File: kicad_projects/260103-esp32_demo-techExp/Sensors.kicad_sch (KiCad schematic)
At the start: 0 parts

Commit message: regular
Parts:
- added C15, C16, C18, C20: 100n, Capacitor_SMD:C_0805_2012Metric, symbol Device:C
- added MK1: CMC-5042PF-AC, esp32_demo_footprints:CUI_CMC-5042PF-AC, symbol CMC-5042PF-AC:CMC-5042PF-AC
- added Q1: TEMT6000X01, esp32_demo_footprints:TRANS_TEMT6000X01, symbol TEMT6000X01:TEMT6000X01
- added R23, R30: 10k, Resistor_SMD:R_0805_2012Metric, symbol Device:R
- added R24, R25: 4k7, Resistor_SMD:R_0805_2012Metric, symbol Device:R
- added R26, R28: 2k, Resistor_SMD:R_0805_2012Metric, symbol Device:R
- added R27, R29: 1M, Resistor_SMD:R_0805_2012Metric, symbol Device:R
- added R31: 100k, Resistor_SMD:R_0805_2012Metric, symbol Device:R
- added U7: BME280, esp32_demo_footprints:PSON65P250X250X100-8N, symbol BME280:BME280
- added U8: MAX4466EXK, esp32_demo_footprints:SOT65P210X110-5N, symbol MAX4466EXK:MAX4466EXK
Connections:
- new net: C16.2, R26.1, R28.2
- new net: MK1.OUT, R27.1, R28.1, R29.2, U8.1 (IN+)
- new net: C20.1, R30.2, R31.1, U8.3 (IN-)
- new net +3.3V: C15.1, C18.1, R23.1, R24.1, R25.1, R26.2, R27.2, U7.2 (CSB), U7.6 (VDDIO), U7.8 (VDD), U8.5 (VCC)
- new net GND: C15.2, C16.1, C18.2, MK1.GND, Q1.1, R29.1, R30.1, U7.1 (GND), U7.5 (SDO), U7.7 (GND), U8.2 (GND)
- new net MIC_OUT: C20.2, R31.2, U8.4 (OUT)
- new net PHOTO_C: Q1.3, R23.2
- new net SCL: R24.2, U7.4 (SCK)
- new net SDA: R25.2, U7.3 (SDI)
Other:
- note added: "BME280"
- note added: "Micophone and amplifier"
- note added: "Photo sensor"
- note added: "for SDO is grounded, the address is 0x76"

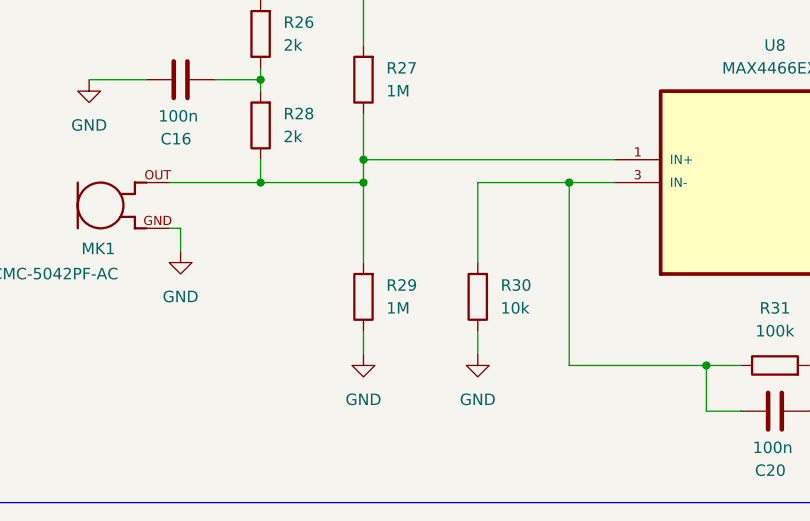
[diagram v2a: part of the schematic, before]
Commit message: regular
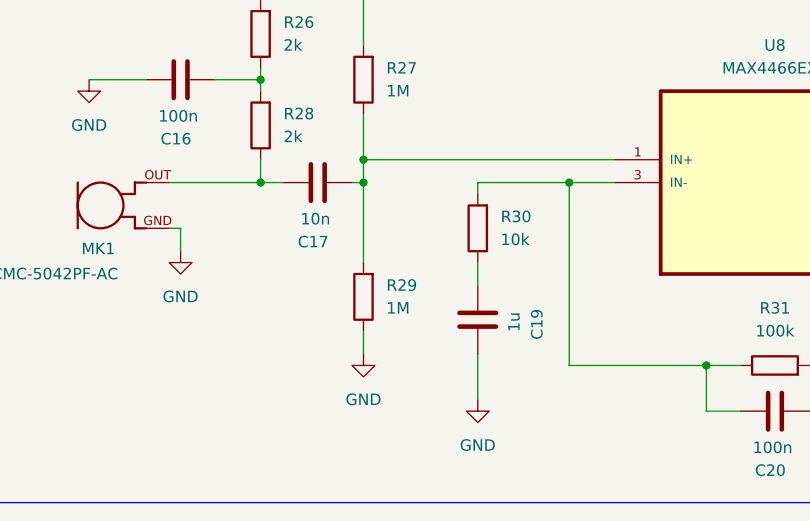
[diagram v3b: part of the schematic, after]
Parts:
- added C17: 10n, Capacitor_SMD:C_0805_2012Metric, symbol Device:C
- added C19: 1u, Capacitor_SMD:C_0805_2012Metric, symbol Device:C
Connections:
- net GND: now also C19.1; no longer R30.1
- net at R27.1, R29.2, U8.1 (IN+): now also C17.2; no longer MK1.OUT, R28.1
- new net: C17.1, MK1.OUT, R28.1
- new net: C19.2, R30.1
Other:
- moved on the sheet: R30
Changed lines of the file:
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@@
+	)
+	(junction
+		(at 176.53 127)
+		(diameter 0)
+		(color 0 0 0 0)
 	)
 	(junction
@@
 	)
 	(junction
-		(at 165.1 127)
-		(diameter 0)
-		(color 0 0 0 0)
-	)
-	(junction
 		(at 250.19 119.38)
 		(diameter 0)
@@
 	)
 	(junction
-		(at 176.53 127)
+		(at 165.1 127)
 		(diameter 0)
 		(color 0 0 0 0)
@@
 	(wire
 		(pts
+			(xy 176.53 127) (xy 176.53 135.89)
+		)
+		(stroke
+			(width 0)
+			(type default)
+		)
+	)
+	(wire
+		(pts
 			(xy 156.21 132.08) (xy 156.21 134.62)
 		)
@@
 	(wire
 		(pts
-			(xy 165.1 127) (xy 176.53 127)
-		)
-		(stroke
-			(width 0)
-			(type default)
-		)
-	)
-	(wire
-		(pts
 			(xy 97.79 54.61) (xy 97.79 52.07)
 		)
@@
 	(wire
 		(pts
-			(xy 189.23 135.89) (xy 189.23 127)
+			(xy 189.23 128.27) (xy 189.23 127)
 		)
 		(stroke
@@
 	(wire
 		(pts
+			(xy 165.1 127) (xy 167.64 127)
+		)
+		(stroke
+			(width 0)
+			(type default)
+		)
+	)
+	(wire
+		(pts
 			(xy 97.79 72.39) (xy 97.79 74.93)
 		)
@@
 	(wire
 		(pts
-			(xy 176.53 127) (xy 176.53 135.89)
-		)
-		(stroke
-			(width 0)
-			(type default)
-		)
-	)
-	(wire
-		(pts
 			(xy 154.94 127) (xy 165.1 127)
 		)
@@
 	(wire
 		(pts
-			(xy 189.23 143.51) (xy 189.23 146.05)
+			(xy 189.23 135.89) (xy 189.23 138.43)
 		)
 		(stroke
@@
 	(wire
 		(pts
+			(xy 189.23 151.13) (xy 189.23 146.05)
+		)
+		(stroke
+			(width 0)
+			(type default)
+		)
+	)
+	(wire
+		(pts
 			(xy 176.53 143.51) (xy 176.53 146.05)
 		)
@@
 		(pts
 			(xy 214.63 152.4) (xy 214.63 147.32)
+		)
+		(stroke
+			(width 0)
+			(type default)
+		)
+	)
+	(wire
+		(pts
+			(xy 175.26 127) (xy 176.53 127)
 		)
 		(stroke
@@
 	(symbol
 		(lib_id "power:GND")
-		(at 189.23 146.05 0)
+		(at 189.23 151.13 0)
 		(unit 1)
 		(exclude_from_sim no)
@@
 		(fields_autoplaced yes)
 		(property "Reference" "#PWR049"
-			(at 189.23 152.4 0)
+			(at 189.23 157.48 0)
 			(effects
 				(font
@@
 		)
 		(property "Value" "GND"
+			(at 189.23 156.21 0)
+			(effects
+				(font
+					(size 1.27 1.27)
+				)
+			)
+		)
+		(property "Footprint" ""
 			(at 189.23 151.13 0)
 			(effects
@@
 					(size 1.27 1.27)
 				)
-			)
-		)
-		(property "Footprint" ""
-			(at 189.23 146.05 0)
-			(effects
-				(font
-					(size 1.27 1.27)
-				)
 				(hide yes)
 			)
 		)
 		(property "Datasheet" ""
-			(at 189.23 146.05 0)
+			(at 189.23 151.13 0)
 			(effects
 				(font
@@
 		)
 		(property "Description" "Power symbol creates a global label with name \"GND\" , ground"
-			(at 189.23 146.05 0)
+			(at 189.23 151.13 0)
 			(effects
 				(font
@@
 	)
 	(symbol
+		(lib_id "Device:C")
+		(at 171.45 127 90)
+		(unit 1)
+		(exclude_from_sim no)
+		(in_bom yes)
+		(on_board yes)
+		(dnp no)
+		(property "Reference" "C17"
+			(at 170.942 133.604 90)
+			(effects
+				(font
+					(size 1.27 1.27)
+				)
+			)
+		)
+		(property "Value" "10n"
+			(at 171.196 131.064 90)
+			(effects
+				(font
+					(size 1.27 1.27)
+				)
+			)
+		)
+		(property "Footprint" "Capacitor_SMD:C_0805_2012Metric"
+			(at 175.26 126.0348 0)
+			(effects
+				(font
+					(size 1.27 1.27)
+				)
+				(hide yes)
+			)
+		)
+		(property "Datasheet" "~"
+			(at 171.45 127 0)
+			(effects
+				(font
+					(size 1.27 1.27)
+				)
+				(hide yes)
+			)
+		)
+		(property "Description" "Unpolarized capacitor"
+			(at 171.45 127 0)
+			(effects
+				(font
+					(size 1.27 1.27)
+				)
+				(hide yes)
+			)
+		)
+		(pin "1"
+		)
+		(pin "2"
+		)
+		(instances
+			(project "260103-esp32_demo-techExp"
+				(path "/2d426d0b-8cb5-4c97-a124-03a3dc3f5ac0/c970ae5e-5c0d-4bfd-b9e3-3da90c7c28e6/aa4b4bc5-e6e9-40a7-8829-625116ed9b5f"
+					(reference "C17")
+					(unit 1)
+				)
+			)
+		)
+	)
+	(symbol
+		(lib_id "Device:C")
+		(at 189.23 142.24 180)
+		(unit 1)
+		(exclude_from_sim no)
+		(in_bom yes)
+		(on_board yes)
+		(dnp no)
+		(property "Reference" "C19"
+			(at 195.834 142.748 90)
+			(effects
+				(font
+					(size 1.27 1.27)
+				)
+			)
+		)
+		(property "Value" "1u"
+			(at 193.294 142.494 90)
+			(effects
+				(font
+					(size 1.27 1.27)
+				)
+			)
+		)
+		(property "Footprint" "Capacitor_SMD:C_0805_2012Metric"
+			(at 188.2648 138.43 0)
+			(effects
+				(font
+					(size 1.27 1.27)
+				)
+				(hide yes)
+			)
+		)
+		(property "Datasheet" "~"
+			(at 189.23 142.24 0)
+			(effects
+				(font
+					(size 1.27 1.27)
+				)
+				(hide yes)
+			)
+		)
+		(property "Description" "Unpolarized capacitor"
+			(at 189.23 142.24 0)
+			(effects
+				(font
+					(size 1.27 1.27)
+				)
+				(hide yes)
+			)
+		)
+		(pin "1"
+		)
+		(pin "2"
+		)
+		(instances
+			(project "260103-esp32_demo-techExp"
+				(path "/2d426d0b-8cb5-4c97-a124-03a3dc3f5ac0/c970ae5e-5c0d-4bfd-b9e3-3da90c7c28e6/aa4b4bc5-e6e9-40a7-8829-625116ed9b5f"
+					(reference "C19")
+					(unit 1)
+				)
+			)
+		)
+	)
+	(symbol
 		(lib_id "Device:R")
 		(at 165.1 120.65 180)
@@
 	(symbol
 		(lib_id "Device:R")
-		(at 189.23 139.7 180)
+		(at 189.23 132.08 180)
 		(unit 1)
 		(exclude_from_sim no)
@@
 		(fields_autoplaced yes)
 		(property "Reference" "R30"
-			(at 191.77 138.4299 0)
+			(at 191.77 130.8099 0)
 			(effects
 				(font
@@
 		)
 		(property "Value" "10k"
-			(at 191.77 140.9699 0)
+			(at 191.77 133.3499 0)
 			(effects
 				(font
@@
 		)
 		(property "Footprint" "Resistor_SMD:R_0805_2012Metric"
-			(at 191.008 139.7 90)
+			(at 191.008 132.08 90)
 			(effects
 				(font
@@
 		)
 		(property "Datasheet" "~"
-			(at 189.23 139.7 0)
+			(at 189.23 132.08 0)
 			(effects
 				(font
@@
 		)
 		(property "Description" "Resistor"
-			(at 189.23 139.7 0)
-			(effects
-				(font
+			(at 189.23 132.08 0)
+			(effects
+				(font
